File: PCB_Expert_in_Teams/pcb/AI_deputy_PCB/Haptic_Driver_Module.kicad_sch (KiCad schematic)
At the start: 23 parts, among them IC1 DA7280-00FVC, IC2 DA7281-00FVC, IC3 DA7282-00FVC, J10 OUTPUT Haptic B (Neck R), J11 OUTPUT Haptic C (Back), J12 Haptic Power and GND, J7 JST CONN from MCU, J9 OUTPUT Haptic A (Neck L)

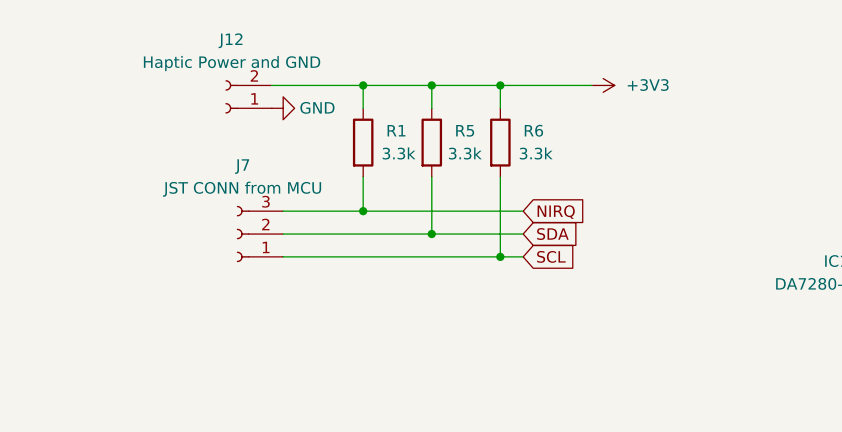
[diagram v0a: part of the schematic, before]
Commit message: update after lab session with gustav saturday
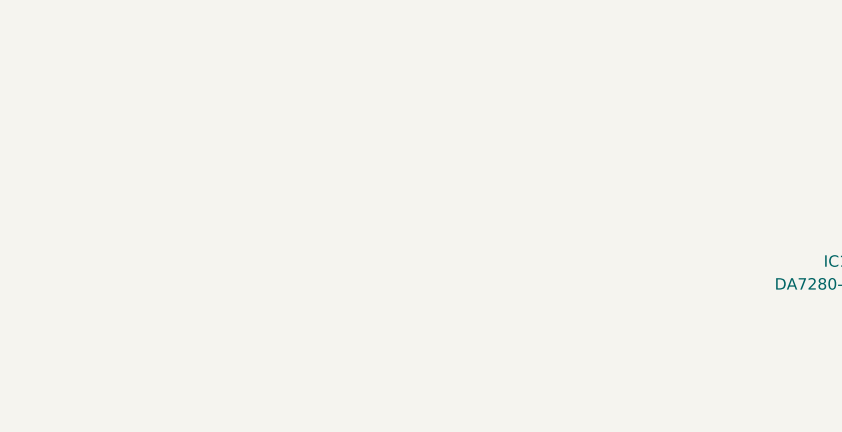
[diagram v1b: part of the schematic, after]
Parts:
- removed J12: Haptic Power and GND, Connector_JST:JST_XH_S2B-XH-A_1x02_P2.50mm_Horizontal, symbol Connector:Conn_01x02_Socket
- removed J7: JST CONN from MCU, Connector_JST:JST_XH_S3B-XH-A_1x03_P2.50mm_Horizontal, symbol Connector:Conn_01x03_Socket
- removed R1, R5, R6: 3.3k, Resistor_SMD:R_0805_2012Metric_Pad1.20x1.40mm_HandSolder, symbol Device:R
